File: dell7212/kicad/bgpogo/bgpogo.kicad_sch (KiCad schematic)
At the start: 5 parts, among them J1 Conn_02x13_Odd_Even, J2 USB1135-15-9-L-B_REVA1, U1 AZ1117-5.0

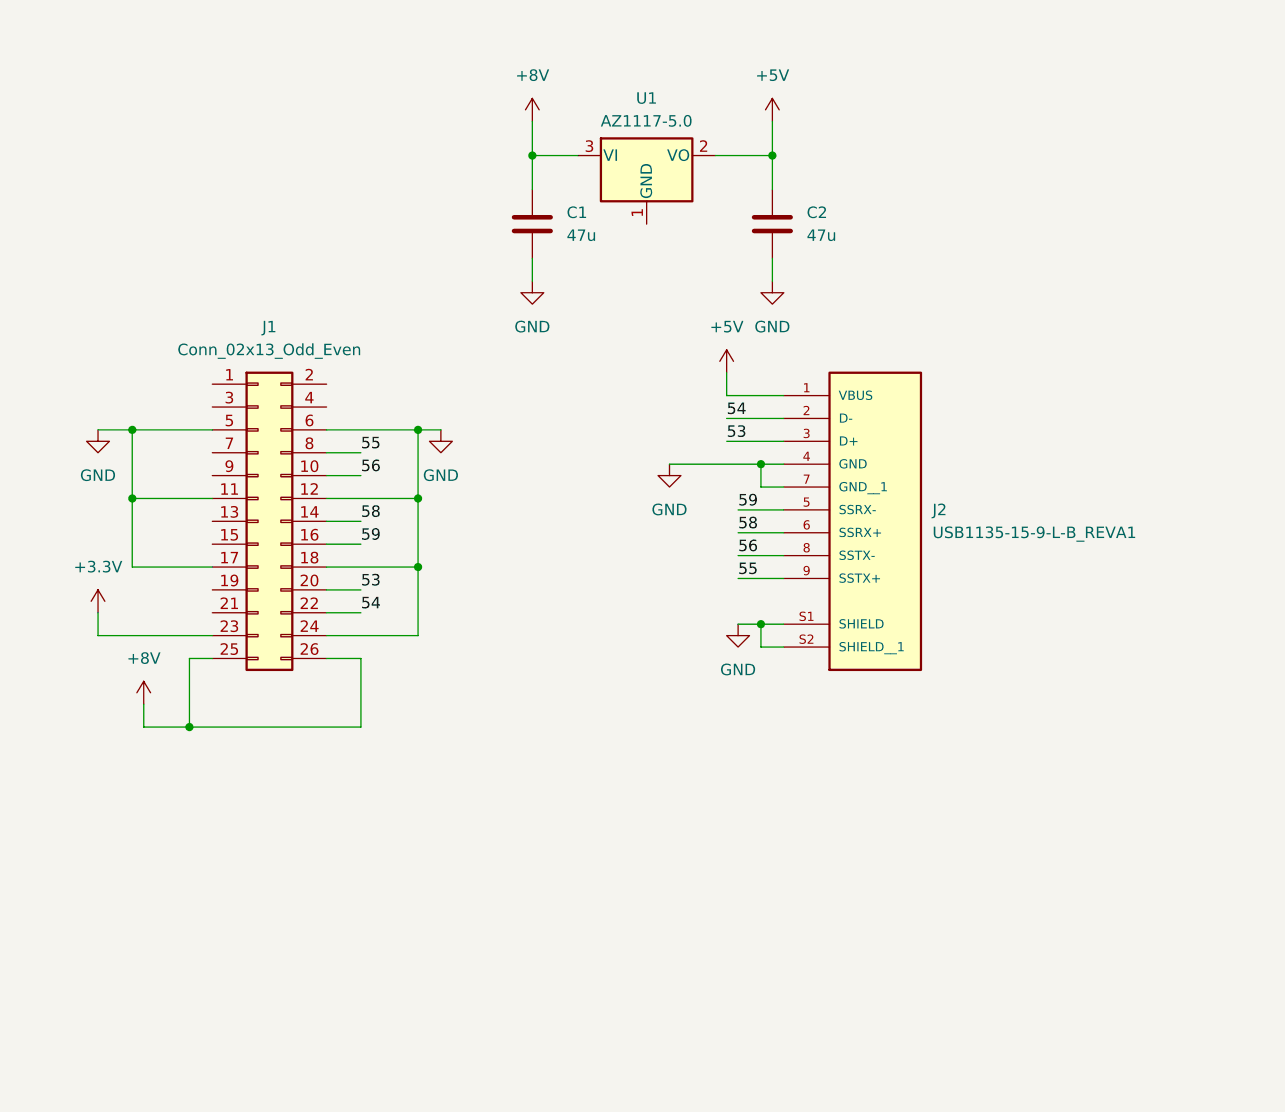
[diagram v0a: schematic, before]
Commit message: pogo sch maybe ready
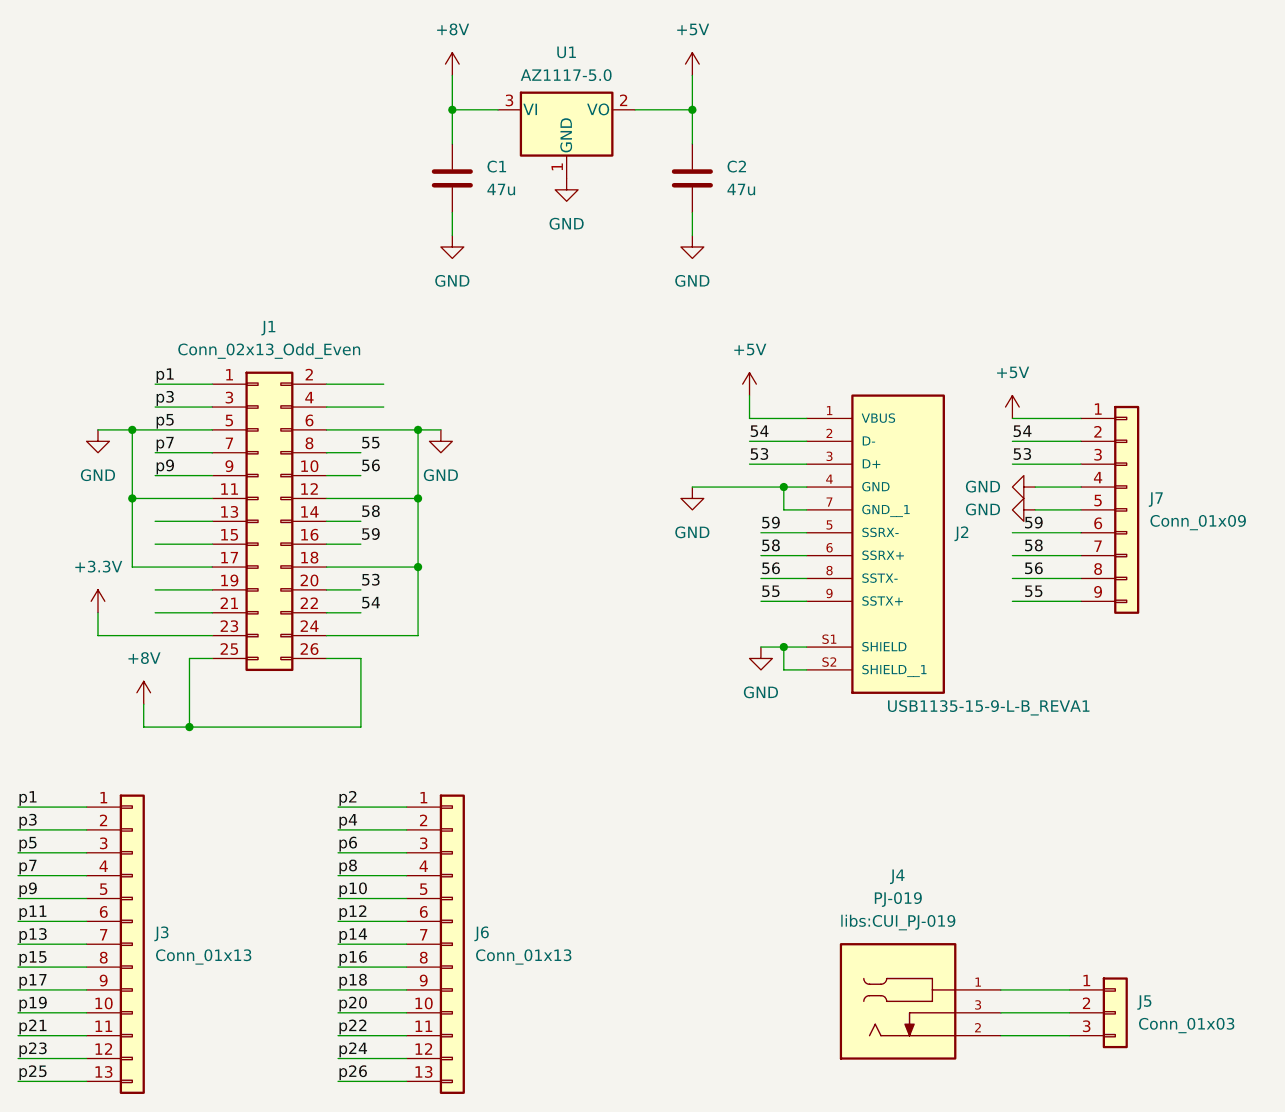
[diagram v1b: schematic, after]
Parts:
- added J3, J6: Conn_01x13, symbol Connector_Generic:Conn_01x13
- added J4: PJ-019, libs:CUI_PJ-019, symbol PJ-019:PJ-019
- added J5: Conn_01x03, symbol Connector_Generic:Conn_01x03
- added J7: Conn_01x09, symbol Connector_Generic:Conn_01x09
- J1: footprint (none) -> pogo1:dell 72xx pogo
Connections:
- net +5V: now also J7.1 (Pin_1)
- net 53: now also J7.3 (Pin_3)
- net 54: now also J7.2 (Pin_2)
- net 55: now also J7.9 (Pin_9)
- net 56: now also J7.8 (Pin_8)
- net 58: now also J7.7 (Pin_7)
- net 59: now also J7.6 (Pin_6)
- net GND: now also U1.1 (GND), J3.3 (Pin_3), J7.4 (Pin_4), J7.5 (Pin_5)
- net p1: now reaches J1.1 (Pin_1)
- net p1: now also J3.1 (Pin_1)
- net p3: now reaches J1.3 (Pin_3)
- net p3: now also J3.2 (Pin_2)
- net p7: now reaches J1.7 (Pin_7)
- net p7: now also J3.4 (Pin_4)
- net p9: now reaches J1.9 (Pin_9)
- net p9: now also J3.5 (Pin_5)
- new net: J4.1, J5.1 (Pin_1)
- new net: J4.2, J5.3 (Pin_3)
- new net: J4.3, J5.2 (Pin_2)
- new net p10: J6.5 (Pin_5)
- new net p11: J3.6 (Pin_6)
- new net p12: J6.6 (Pin_6)
- new net p13: J3.7 (Pin_7)
- new net p14: J6.7 (Pin_7)
- new net p15: J3.8 (Pin_8)
- new net p16: J6.8 (Pin_8)
- new net p17: J3.9 (Pin_9)
- new net p18: J6.9 (Pin_9)
- new net p19: J3.10 (Pin_10)
- new net p2: J6.1 (Pin_1)
- new net p20: J6.10 (Pin_10)
- new net p21: J3.11 (Pin_11)
- new net p22: J6.11 (Pin_11)
- new net p23: J3.12 (Pin_12)
- new net p24: J6.12 (Pin_12)
- new net p25: J3.13 (Pin_13)
- new net p26: J6.13 (Pin_13)
- new net p4: J6.2 (Pin_2)
- new net p6: J6.3 (Pin_3)
- new net p8: J6.4 (Pin_4)
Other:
- moved on the sheet: C1, C2, J2, U1

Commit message: pogo sch assign header footprints.
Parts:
- J5: footprint (none) -> Connector_PinHeader_2.54mm:PinHeader_1x03_P2.54mm_Vertical
- J6: footprint (none) -> Connector_PinHeader_2.54mm:PinHeader_1x13_P2.54mm_Vertical
- J7: footprint (none) -> Connector_PinHeader_2.54mm:PinHeader_1x09_P2.54mm_Vertical
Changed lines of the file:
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@@
 			)
 		)
-		(property "Footprint" ""
+		(property "Footprint" "Connector_PinHeader_2.54mm:PinHeader_1x09_P2.54mm_Vertical"
 			(at 149.86 74.93 0)
 			(effects
@@
 			)
 		)
-		(property "Footprint" ""
+		(property "Footprint" "Connector_PinHeader_2.54mm:PinHeader_1x13_P2.54mm_Vertical"
 			(at 74.93 123.19 0)
 			(effects
@@
 			)
 		)
-		(property "Footprint" ""
+		(property "Footprint" "Connector_PinHeader_2.54mm:PinHeader_1x03_P2.54mm_Vertical"
 			(at 148.59 130.81 0)
 			(effects
